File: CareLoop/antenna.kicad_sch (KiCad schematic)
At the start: 5 parts, among them J1 Conn_Coaxial_Small

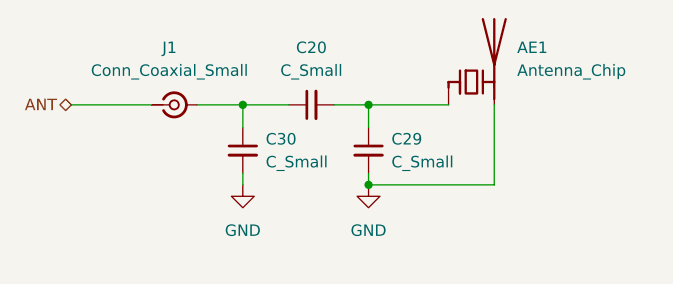
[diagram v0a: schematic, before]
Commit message: updated antenna version
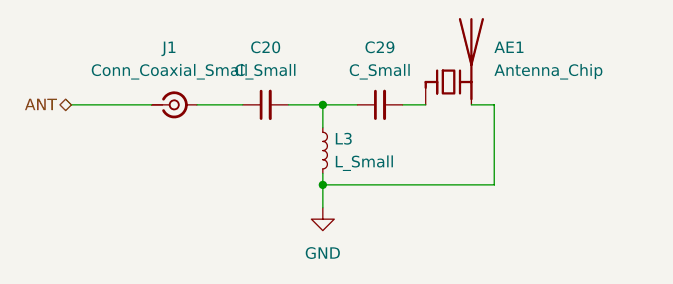
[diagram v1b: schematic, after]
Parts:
- removed C30: C_Small, Capacitor_SMD:C_0603_1608Metric_Pad1.08x0.95mm_HandSolder, symbol Device:C_Small
- added L3: L_Small, symbol Device:L_Small
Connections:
- net GND: now also L3.2; no longer C29.2
- net at C20.2, C29.1: now also L3.1; no longer AE1.1 (FEED)
- new net: AE1.1 (FEED), C29.2
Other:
- moved on the sheet: C20
